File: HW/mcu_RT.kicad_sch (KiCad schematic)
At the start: 33 parts, among them U41 STM32G474VETx, U44 LM1084-5.0, U45 LM1084-3.3, Y1 Crystal_GND24

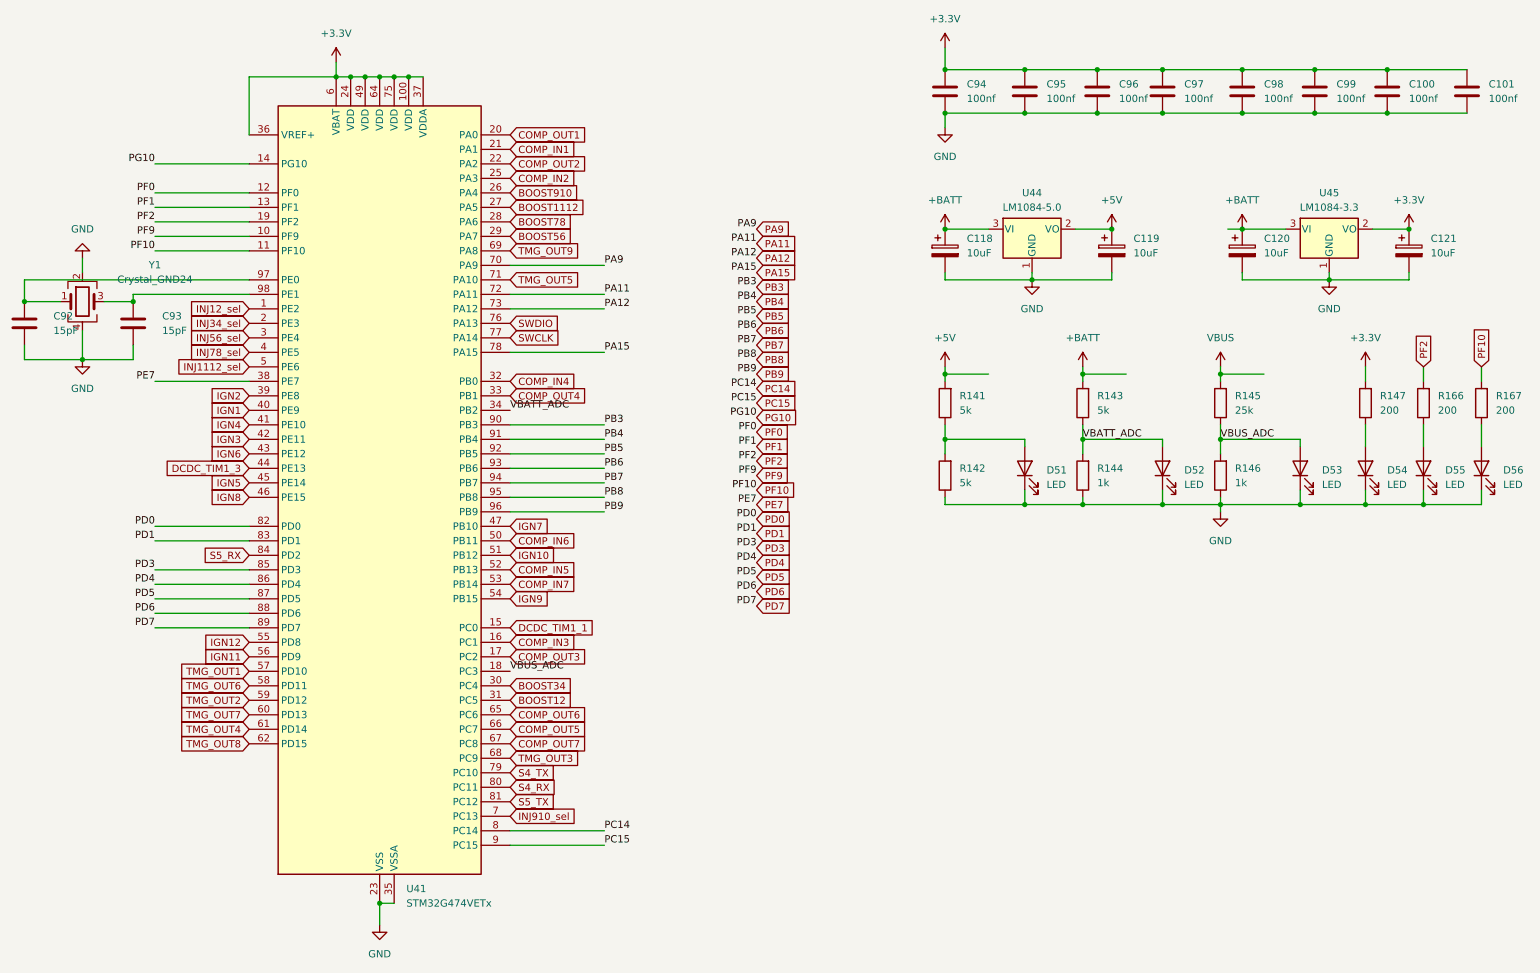
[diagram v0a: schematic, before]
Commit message: Ver2
Second HW rev + SW update
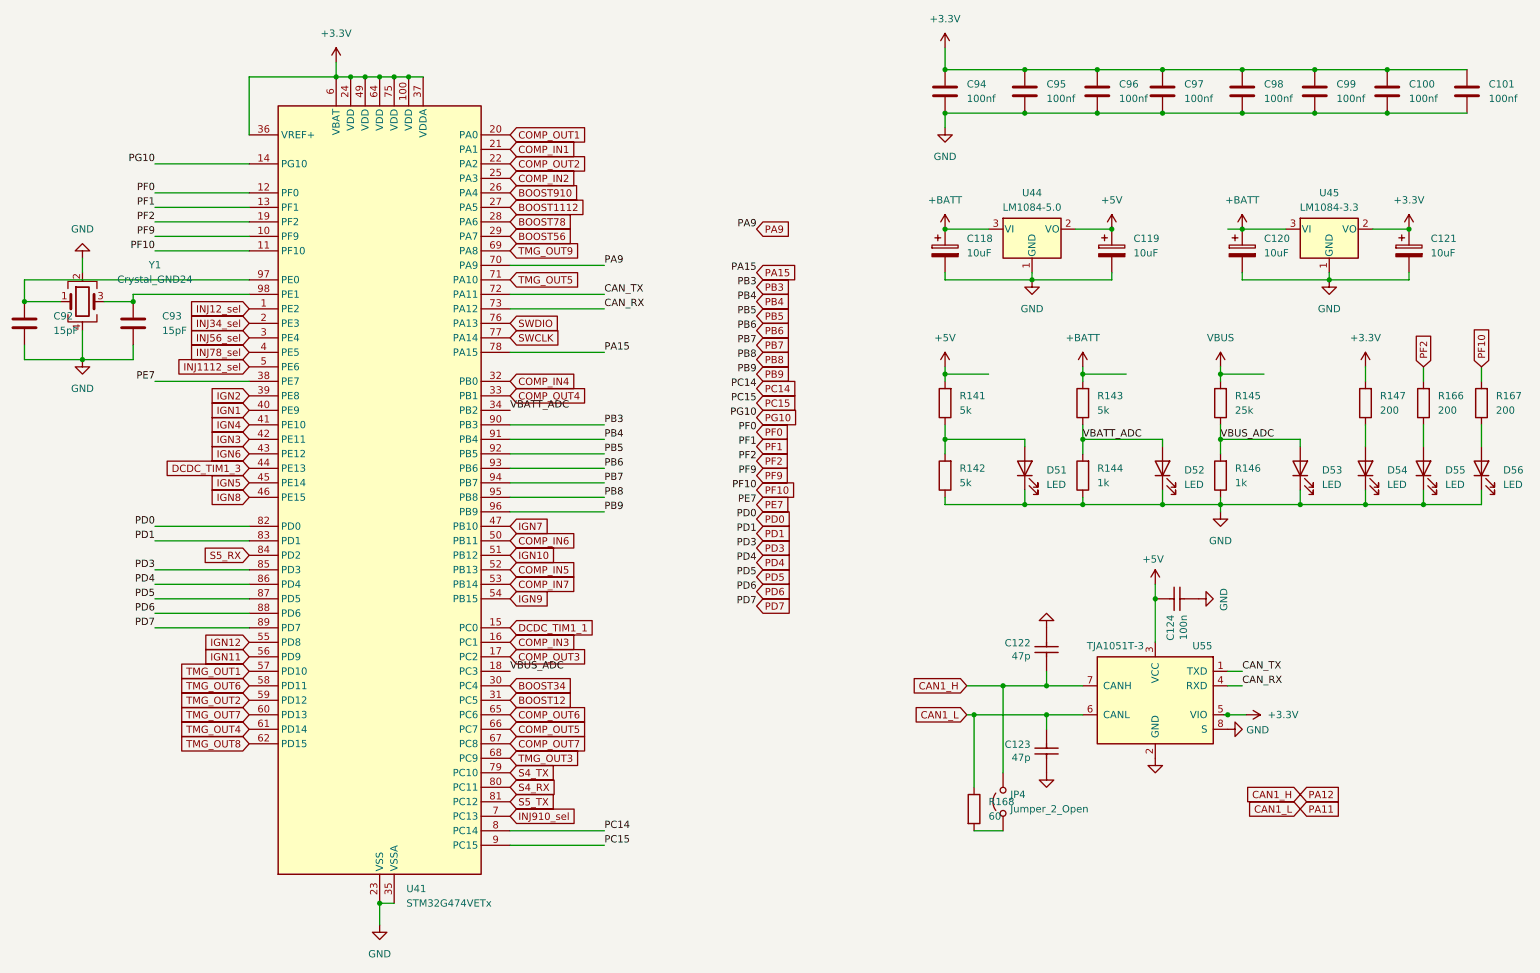
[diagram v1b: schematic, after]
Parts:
- added C122, C123: 47p, Capacitor_SMD:C_0402_1005Metric, symbol hellen-one-common:Cap
- added C124: 100n, Capacitor_SMD:C_0402_1005Metric, symbol hellen-one-common:Cap
- added JP4: Jumper_2_Open, Jumper:SolderJumper-2_P1.3mm_Open_RoundedPad1.0x1.5mm, symbol Jumper:Jumper_2_Open
- added R168: 60, Resistor_SMD:R_0402_1005Metric, symbol Device:R
- added U55: TJA1051T-3, Package_SO:SOIC-8_3.9x4.9mm_P1.27mm, symbol Interface_CAN_LIN:TJA1051T-3
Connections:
- net +3.3V: now also U55.5 (VIO)
- net +5V: now also C124.2, U55.3 (VCC)
- net GND: now also C122.2, C123.1, C124.1, U55.2 (GND), U55.8 (S)
- net PA11 renamed CAN_TX
- net CAN_TX: now also U55.1 (TXD)
- net PA12 renamed CAN_RX
- net CAN_RX: now also U55.4 (RXD)
- new net: JP4.1 (A), R168.2
- new net CAN1_H: C122.1, JP4.2 (B), U55.7 (CANH)
- new net CAN1_L: C123.2, R168.1, U55.6 (CANL)
